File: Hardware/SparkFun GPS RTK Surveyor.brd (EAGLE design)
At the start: 69.1 x 110.1 mm, 196 parts, among them J13 Internal, J16 microSD, J17 Qwiic Right Angle, J3 USB Female Type C Connector, J4 External, J5 USB Female Type C Connector, J6 Start Base, J7 Power Switch, Q2 MBT3904DW1T1, U10 MCP73833, U2 3.3V, U3 U-BLOX_ZED-F9P, U4 3.3V, U5 ESP-WROOM-32NARROW, U6 CH340C, U7 MAX17048

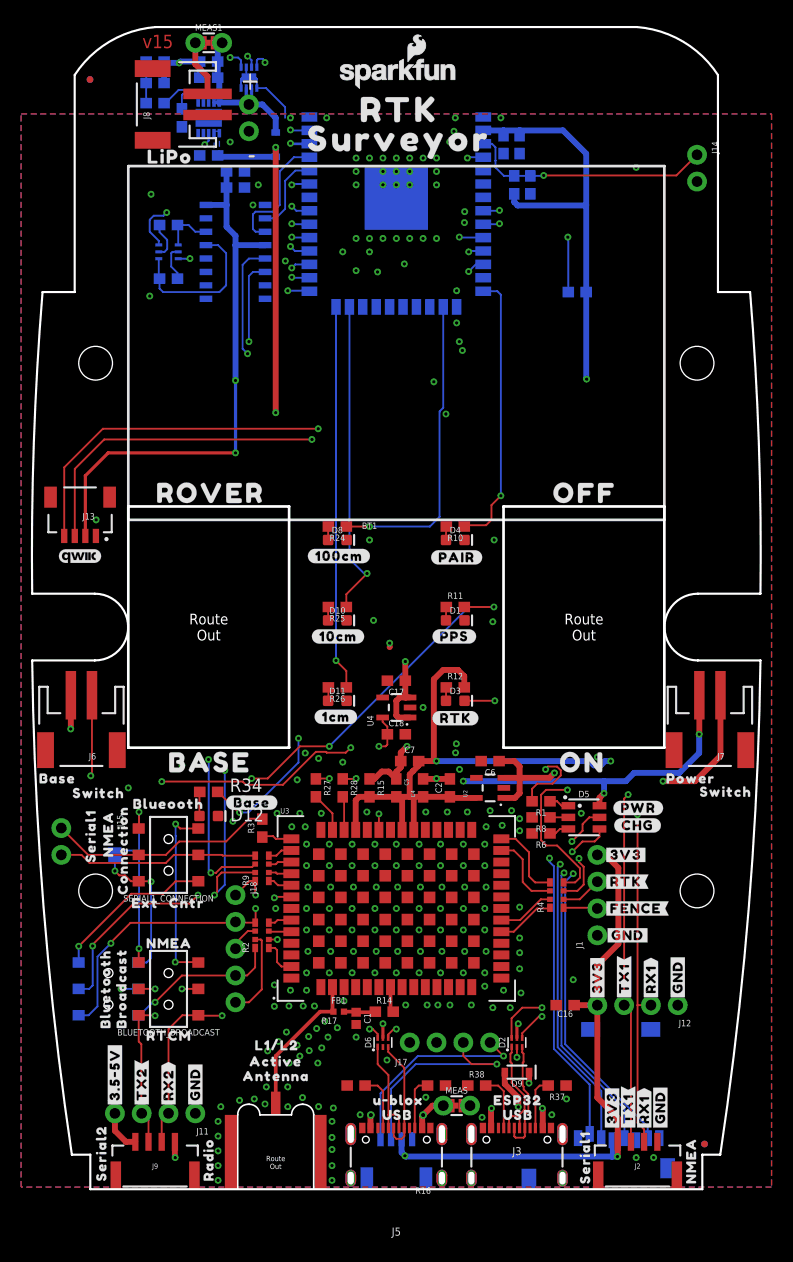
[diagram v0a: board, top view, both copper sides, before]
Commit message: 2x2 Panel
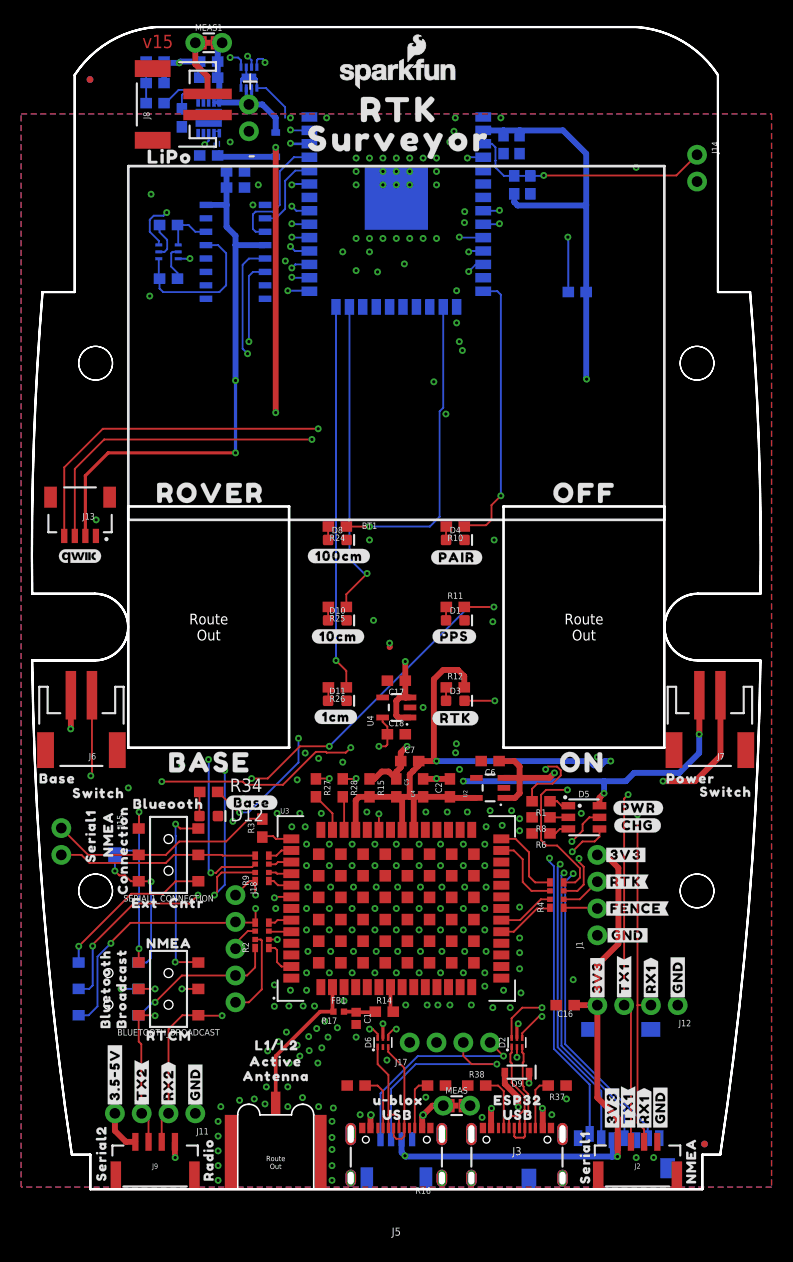
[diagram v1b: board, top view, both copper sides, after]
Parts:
- moved U$2 10.2 mm to (73.7, 81.3)
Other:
- outline, holes or cut-outs redrawn
- board text added: "Connectors"
- board text added: "Face to Lid LEDs this side"
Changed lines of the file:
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@@
 <layers>
 <layer number="1" name="Top" color="4" fill="1" visible="yes" active="yes"/>
-<layer number="2" name="Horz/GND" color="1" fill="3" visible="no" active="yes"/>
-<layer number="15" name="Vert" color="4" fill="6" visible="no" active="yes"/>
+<layer number="2" name="Horz/GND" color="1" fill="3" visible="yes" active="yes"/>
+<layer number="15" name="Vert" color="4" fill="6" visible="yes" active="yes"/>
 <layer number="16" name="Bottom" color="1" fill="1" visible="yes" active="yes"/>
 <layer number="17" name="Pads" color="2" fill="1" visible="yes" active="yes"/>
@@
 <layer number="23" name="tOrigins" color="15" fill="1" visible="yes" active="yes"/>
 <layer number="24" name="bOrigins" color="15" fill="1" visible="yes" active="yes"/>
-<layer number="25" name="tNames" color="7" fill="1" visible="no" active="yes"/>
-<layer number="26" name="bNames" color="7" fill="1" visible="no" active="yes"/>
-<layer number="27" name="tValues" color="7" fill="1" visible="no" active="yes"/>
-<layer number="28" name="bValues" color="7" fill="1" visible="no" active="yes"/>
-<layer number="29" name="tStop" color="7" fill="3" visible="no" active="yes"/>
-<layer number="30" name="bStop" color="7" fill="6" visible="no" active="yes"/>
-<layer number="31" name="tCream" color="7" fill="4" visible="no" active="yes"/>
-<layer number="32" name="bCream" color="7" fill="5" visible="no" active="yes"/>
-<layer number="33" name="tFinish" color="6" fill="3" visible="no" active="yes"/>
-<layer number="34" name="bFinish" color="6" fill="6" visible="no" active="yes"/>
-<layer number="35" name="tGlue" color="7" fill="4" visible="no" active="yes"/>
-<layer number="36" name="bGlue" color="7" fill="5" visible="no" active="yes"/>
-<layer number="37" name="tTest" color="7" fill="1" visible="no" active="yes"/>
-<layer number="38" name="bTest" color="7" fill="1" visible="no" active="yes"/>
-<layer number="39" name="tKeepout" color="4" fill="11" visible="no" active="yes"/>
-<layer number="40" name="bKeepout" color="1" fill="11" visible="no" active="yes"/>
-<layer number="41" name="tRestrict" color="4" fill="10" visible="no" active="yes"/>
-<layer number="42" name="bRestrict" color="1" fill="10" visible="no" active="yes"/>
-<layer number="43" name="vRestrict" color="2" fill="10" visible="no" active="yes"/>
-<layer number="44" name="Drills" color="7" fill="1" visible="no" active="yes"/>
+<layer number="25" name="tNames" color="7" fill="1" visible="yes" active="yes"/>
+<layer number="26" name="bNames" color="7" fill="1" visible="yes" active="yes"/>
+<layer number="27" name="tValues" color="7" fill="1" visible="yes" active="yes"/>
+<layer number="28" name="bValues" color="7" fill="1" visible="yes" active="yes"/>
+<layer number="29" name="tStop" color="7" fill="3" visible="yes" active="yes"/>
+<layer number="30" name="bStop" color="7" fill="6" visible="yes" active="yes"/>
+<layer number="31" name="tCream" color="7" fill="4" visible="yes" active="yes"/>
+<layer number="32" name="bCream" color="7" fill="5" visible="yes" active="yes"/>
+<layer number="33" name="tFinish" color="6" fill="3" visible="yes" active="yes"/>
+<layer number="34" name="bFinish" color="6" fill="6" visible="yes" active="yes"/>
+<layer number="35" name="tGlue" color="7" fill="4" visible="yes" active="yes"/>
+<layer number="36" name="bGlue" color="7" fill="5" visible="yes" active="yes"/>
+<layer number="37" name="tTest" color="7" fill="1" visible="yes" active="yes"/>
+<layer number="38" name="bTest" color="7" fill="1" visible="yes" active="yes"/>
+<layer number="39" name="tKeepout" color="4" fill="11" visible="yes" active="yes"/>
+<layer number="40" name="bKeepout" color="1" fill="11" visible="yes" active="yes"/>
+<layer number="41" name="tRestrict" color="4" fill="10" visible="yes" active="yes"/>
+<layer number="42" name="bRestrict" color="1" fill="10" visible="yes" active="yes"/>
+<layer number="43" name="vRestrict" color="2" fill="10" visible="yes" active="yes"/>
+<layer number="44" name="Drills" color="7" fill="1" visible="yes" active="yes"/>
 <layer number="45" name="Holes" color="7" fill="1" visible="yes" active="yes"/>
-<layer number="46" name="Milling" color="3" fill="1" visible="no" active="yes"/>
-<layer number="47" name="Measures" color="7" fill="1" visible="no" active="yes"/>
-<layer number="48" name="Document" color="7" fill="1" visible="no" active="yes"/>
+<layer number="46" name="Milling" color="3" fill="1" visible="yes" active="yes"/>
+<layer number="47" name="Measures" color="7" fill="1" visible="yes" active="yes"/>
+<layer number="48" name="Document" color="7" fill="1" visible="yes" active="yes"/>
 <layer number="49" name="Reference" color="7" fill="1" visible="yes" active="yes"/>
-<layer number="50" name="dxf" color="7" fill="1" visible="no" active="yes"/>
+<layer number="50" name="dxf" color="7" fill="1" visible="yes" active="yes"/>
 <layer number="51" name="tDocu" color="6" fill="1" visible="yes" active="yes"/>
-<layer number="52" name="bDocu" color="7" fill="1" visible="no" active="yes"/>
+<layer number="52" name="bDocu" color="7" fill="1" visible="yes" active="yes"/>
 <layer number="91" name="Nets" color="2" fill="1" visible="no" active="no"/>
 <layer number="92" name="Busses" color="1" fill="1" visible="no" active="no"/>
@@
 <plain>
 <text x="2.794" y="108.839" size="1.27" layer="1" font="vector" ratio="15" rot="SR0" align="center">v15</text>
-<text x="64.77" y="68.58" size="1.778" layer="51" font="vector" ratio="15">Board thickness is 1.6mm</text>
-<text x="64.77" y="63.5" size="1.778" layer="51" font="vector" ratio="15">No clean process</text>
-<text x="64.77" y="66.04" size="1.778" layer="51" font="vector" ratio="15">4 Layer Board</text>
+<text x="74.93" y="68.58" size="1.778" layer="51" font="vector" ratio="15">Board thickness is 1.6mm</text>
+<text x="74.93" y="63.5" size="1.778" layer="51" font="vector" ratio="15">No clean process</text>
+<text x="74.93" y="66.04" size="1.778" layer="51" font="vector" ratio="15">4 Layer Board</text>
 <circle x="26.11" y="9.27" radius="1.5" width="0.1" layer="48"/>
 <circle x="31.11" y="9.27" radius="1.5" width="0.1" layer="48"/>
@@
 <dimension x1="-9.144" y1="56.515" x2="59.944" y2="56.007" x3="25.4" y3="116.84" textsize="1.016" textratio="15" layer="47" dtype="horizontal" width="0.0762"/>
 <dimension x1="-11.684" y1="110.617" x2="-10.668" y2="0.111" x3="-11.557" y3="55.364" textsize="1.016" textratio="15" layer="47" dtype="vertical" width="0.0762"/>
+<text x="25.4" y="6.54" size="0.5" layer="51" ratio="20" align="center">Face to Lid
+LEDs this side</text>
+<text x="25.4" y="2" size="0.5" layer="51" ratio="20" rot="R180" align="center">Connectors</text>
+<wire x1="2.5908" y1="110.205" x2="48.2092" y2="110.205" width="0.2032" layer="20"/>
+<hole x="-3.0988" y="28.3337" drill="3.2004"/>
+<hole x="-3.0988" y="78.3463" drill="3.2004"/>
+<hole x="53.8988" y="78.3463" drill="3.2004"/>
+<hole x="53.8988" y="28.3337" drill="3.2004"/>
+<wire x1="-9.1092" y1="50.1777" x2="-3.175" y2="50.1777" width="0.2032" layer="20"/>
+<wire x1="-3.175" y1="56.5023" x2="-9.1092" y2="56.5023" width="0.2032" layer="20"/>
+<wire x1="-6.3119" y1="102.87" x2="2.5908" y2="110.205" width="0.2032" layer="51" curve="-72.045824"/>
+<wire x1="-9.1092" y1="56.5023" x2="-6.3119" y2="102.87" width="0.2032" layer="51" curve="-8.331372"/>
+<wire x1="-3.175" y1="50.1777" x2="-3.175" y2="56.5023" width="0.2032" layer="20" curve="180"/>
+<wire x1="59.9092" y1="50.1777" x2="53.975" y2="50.1777" width="0.2032" layer="20"/>
+<wire x1="53.975" y1="56.5023" x2="59.9092" y2="56.5023" width="0.2032" layer="20"/>
+<wire x1="53.975" y1="50.1777" x2="53.975" y2="56.5023" width="0.2032" layer="20" curve="-180"/>
+<wire x1="-8.128" y1="85.09" x2="-5.08" y2="85.09" width="0.2032" layer="20"/>
+<wire x1="-5.08" y1="85.09" x2="-5.08" y2="105.664" width="0.2032" layer="20"/>
+<wire x1="-9.1092" y1="56.5023" x2="-8.128" y2="85.09" width="0.2032" layer="20" curve="-5.381392"/>
+<wire x1="-5.08" y1="105.664" x2="2.5908" y2="110.205" width="0.2032" layer="20" curve="-52.405474"/>
+<wire x1="-3.6" y1="0.065" x2="54.4" y2="0.065" width="0.2032" layer="20"/>
+<wire x1="-3.6" y1="0.065" x2="-3.6" y2="3.34" width="0.2032" layer="20"/>
+<wire x1="-3.6" y1="3.34" x2="-5.35" y2="3.34" width="0.2032" layer="20"/>
+<wire x1="54.4" y1="0.065" x2="54.4" y2="3.34" width="0.2032" layer="20"/>
+<wire x1="54.4" y1="3.34" x2="56.1" y2="3.34" width="0.2032" layer="20"/>
+<wire x1="-5.35" y1="3.34" x2="-9.1092" y2="50.1777" width="0.2032" layer="20" curve="-7.756885"/>
+<wire x1="56.1" y1="3.34" x2="59.9092" y2="50.1777" width="0.2032" layer="20" curve="7.756885"/>
+<wire x1="57.1119" y1="102.87" x2="48.2092" y2="110.205" width="0.2032" layer="51" curve="72.045824"/>
+<wire x1="59.9092" y1="56.5023" x2="57.1119" y2="102.87" width="0.2032" layer="51" curve="8.331372"/>
+<wire x1="58.928" y1="85.09" x2="55.88" y2="85.09" width="0.2032" layer="20"/>
+<wire x1="55.88" y1="85.09" x2="55.88" y2="105.664" width="0.2032" layer="20"/>
+<wire x1="59.9092" y1="56.5023" x2="58.928" y2="85.09" width="0.2032" layer="20" curve="5.381392"/>
+<wire x1="55.88" y1="105.664" x2="48.2092" y2="110.205" width="0.2032" layer="20" curve="52.405474"/>
 </plain>
 <attributes>
@@
 <attribute name="PROD_ID" value="CONN-14122" x="25.4" y="6.207" size="1.778" layer="27" display="off"/>
 </element>
-<element name="U$2" library="SparkFun-Aesthetics" package="ORDERING_INSTRUCTIONS" value="SPECIAL_INSTRUCTIONS-ORDERING" x="63.5" y="81.28" smashed="yes"/>
+<element name="U$2" library="SparkFun-Aesthetics" package="ORDERING_INSTRUCTIONS" value="SPECIAL_INSTRUCTIONS-ORDERING" x="73.66" y="81.28" smashed="yes"/>
 <element name="C2" library="SparkFun-Capacitors" package="0603" value="1.0uF" x="30.48" y="38.1" smashed="yes" rot="R90">
 <attribute name="NAME" x="29.718" y="38.1" size="0.6096" layer="25" font="vector" ratio="20" rot="R90" align="bottom-center"/>
